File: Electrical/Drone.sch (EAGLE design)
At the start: 76 parts, among them IC1 EFM8BB21F16G-C-QFN20R, IC2 FD6288Q, IC3 LDL212PV33R, IC4 LDL212PV33R, IC5 LDL212PV33R, IC6 LDL212PV33R, J1 GSB1C41110SSHR, Q10 SSM6K504NU, Q11 SSM6K504NU, Q6 SSM6K504NU, Q7 SSM6K504NU, Q8 SSM6K504NU, Q9 SSM6K504NU, U1 TPSM863252RDXR, U2 ESP32-S3-PICO-1-N8R2

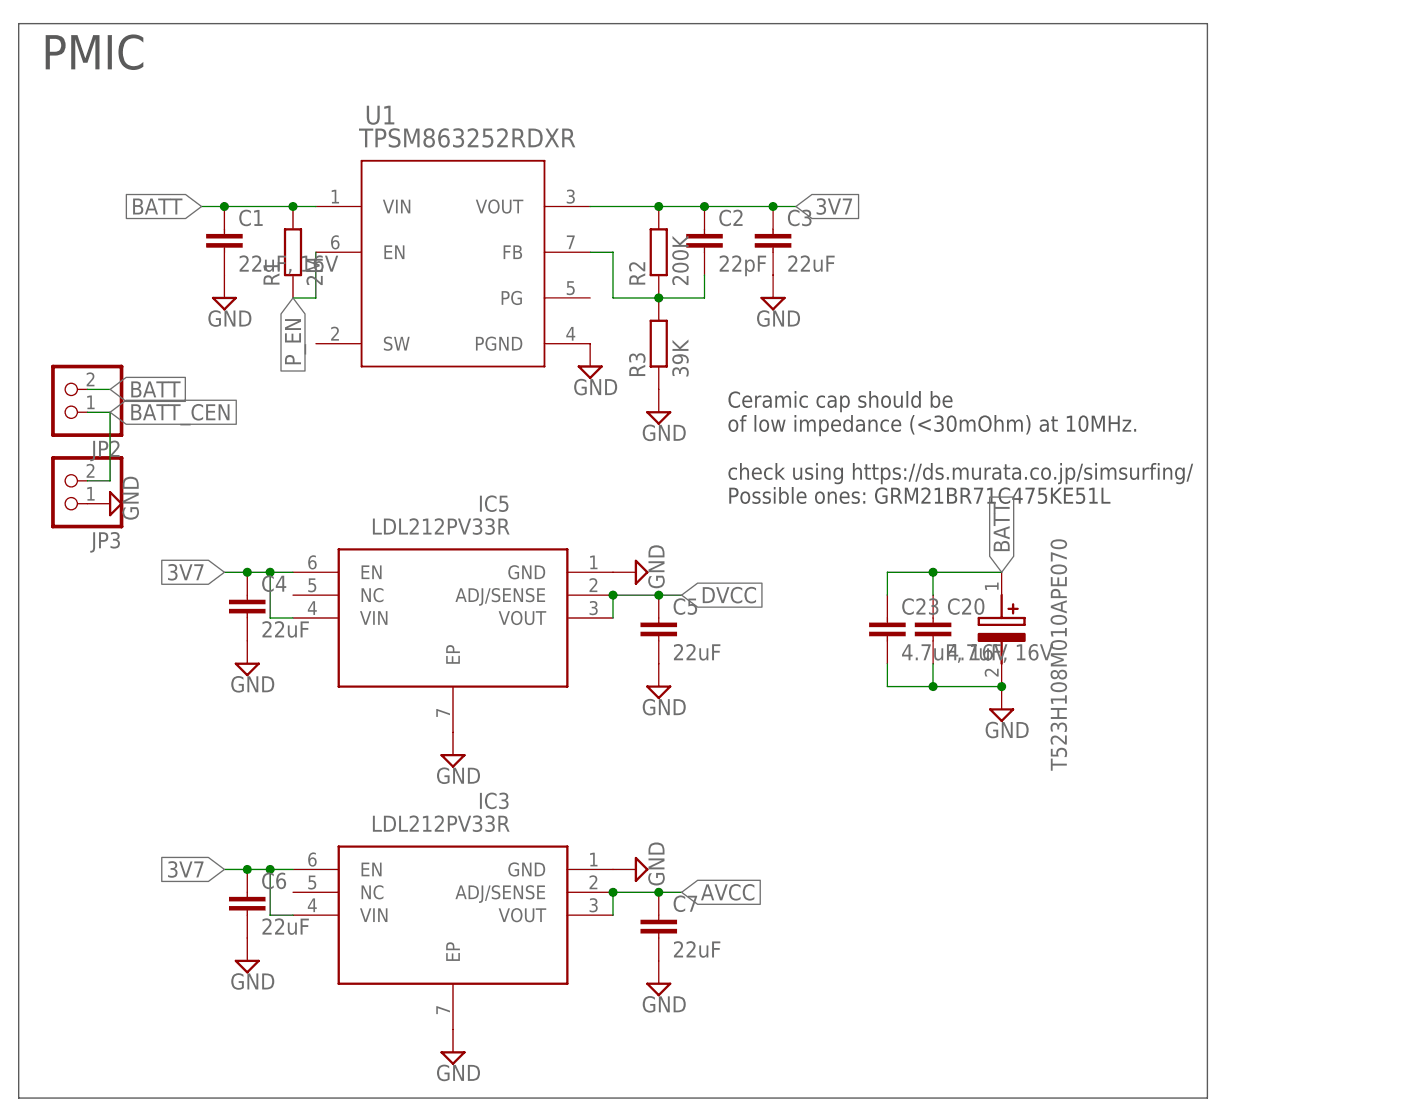
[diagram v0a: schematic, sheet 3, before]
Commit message: Simplify PCB design
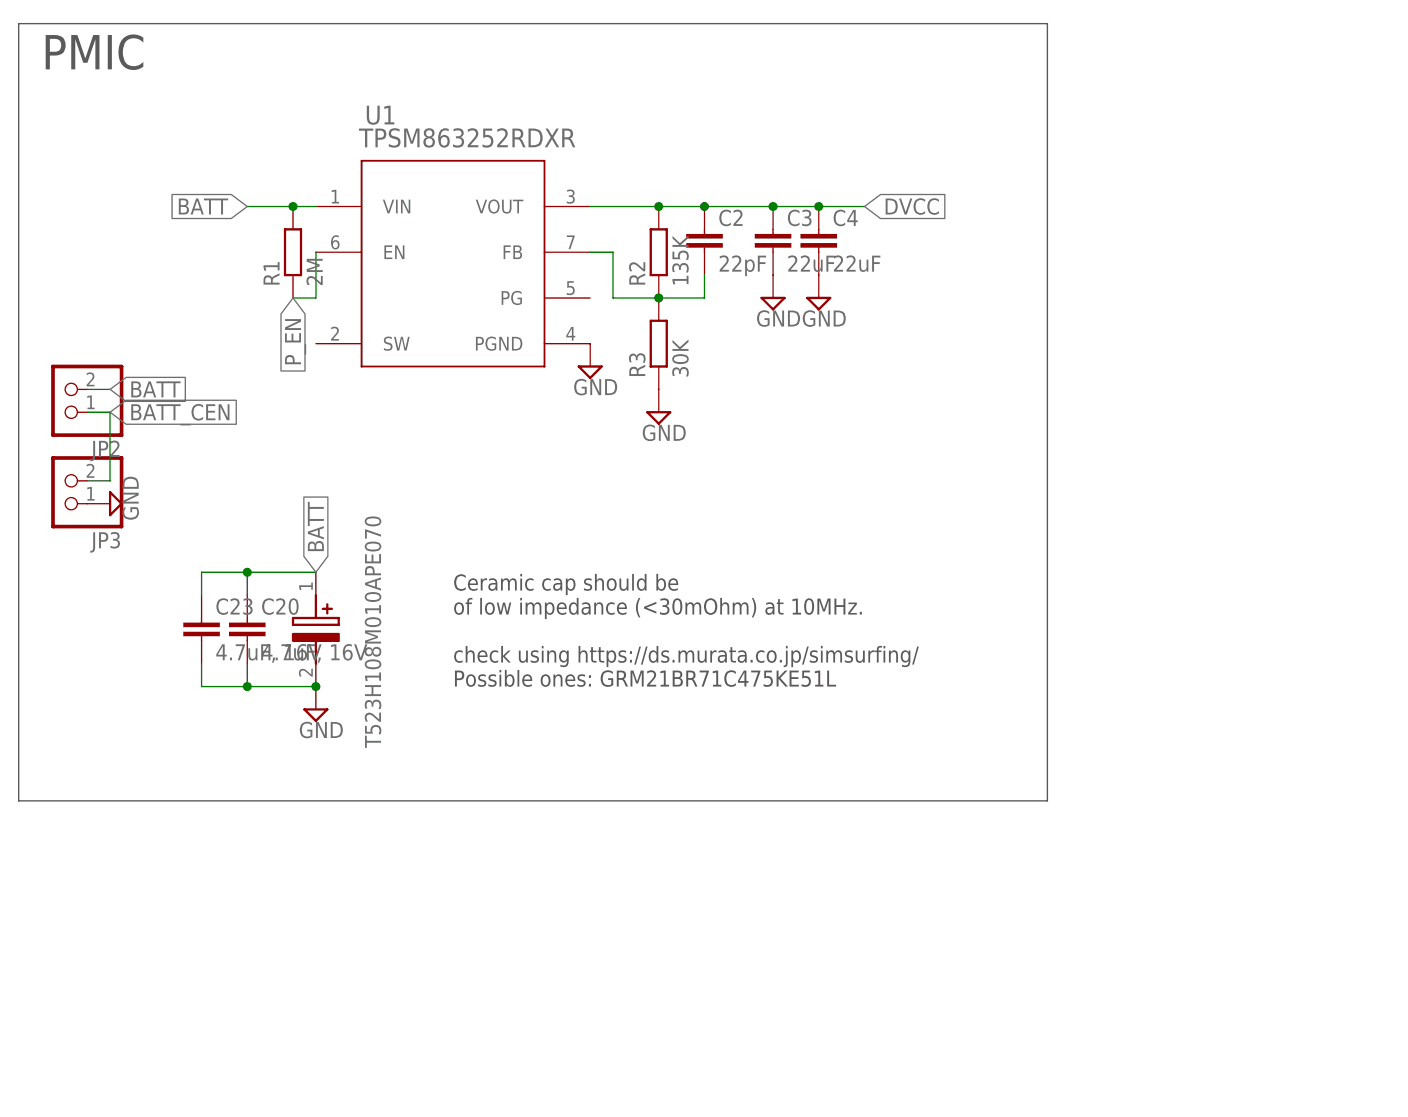
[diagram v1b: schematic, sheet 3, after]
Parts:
- removed C1: 22uF, 16V, rcl:C-EUC0603
- removed C5, C6, C7: 22uF, rcl:C-EUC0603
- removed IC3, IC5: LDL212PV33R, SamacSys_Parts:LDL212PV33R
- R2: value 200K -> 135K
- R3: value 39K -> 30K
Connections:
- removed net 3V7: C2.1, C3.1, C4.1, C6.1, IC3.EN, IC3.VIN, IC5.EN, IC5.VIN, R2.2, U1.VOUT
- removed net AVCC: C7.1, IC3.ADJ/SENSE, IC3.VOUT
- net BATT: no longer C1.1
- net DVCC: now also C2.1, C3.1, C4.1, R2.2, U1.VOUT; no longer C5.1, IC5.ADJ/SENSE, IC5.VOUT
- net GND: no longer C1.2, C5.2, C6.2, C7.2, IC3.EP, IC3.GND, IC5.EP, IC5.GND
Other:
- moved on the sheet: C20, C23, C4
